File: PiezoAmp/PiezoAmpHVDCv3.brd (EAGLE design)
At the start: 82.5 x 101.3 mm, 35 parts, among them IC1 LM101N, Q1 IRF512, Q2 IRF512, Q3 2N3904, U1 RXX100, X1 MAB32

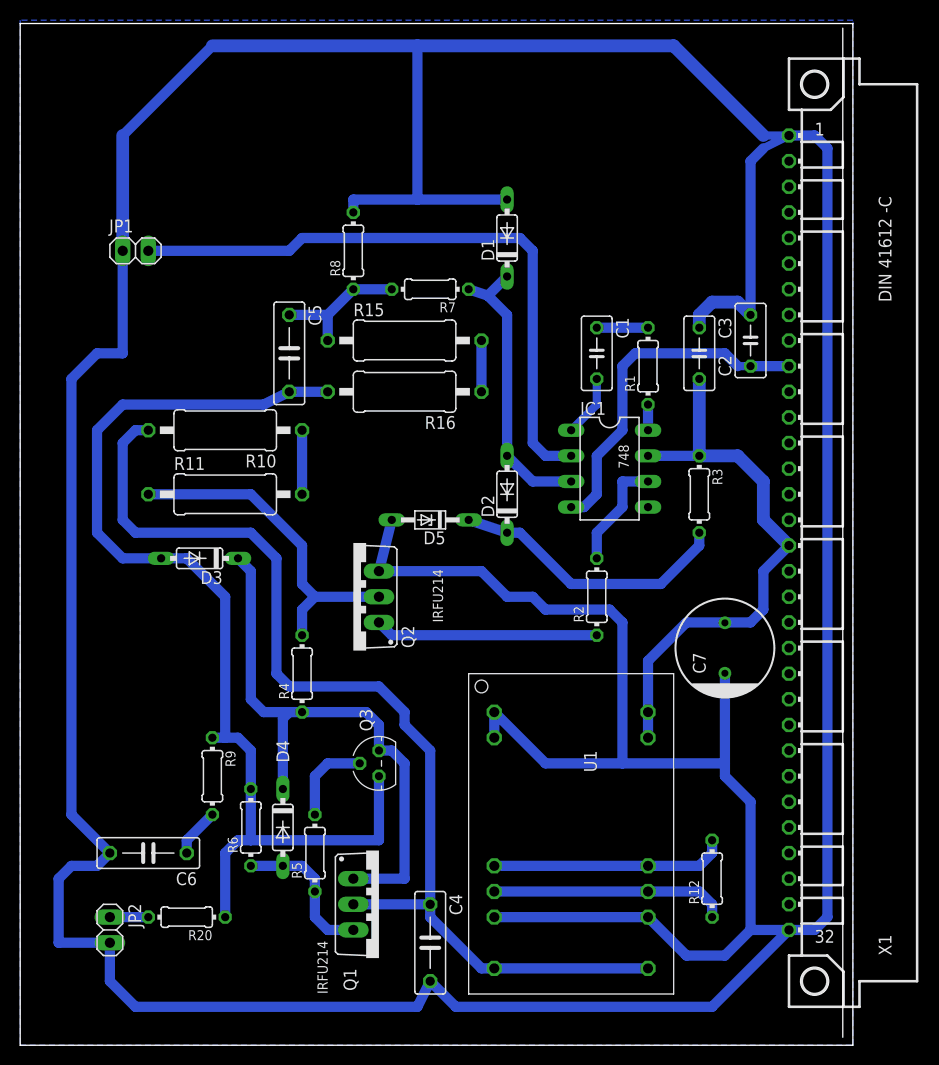
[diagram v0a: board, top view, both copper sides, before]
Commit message: Trying to clean up
Clean up, add Piezo sent to DirtyPCB
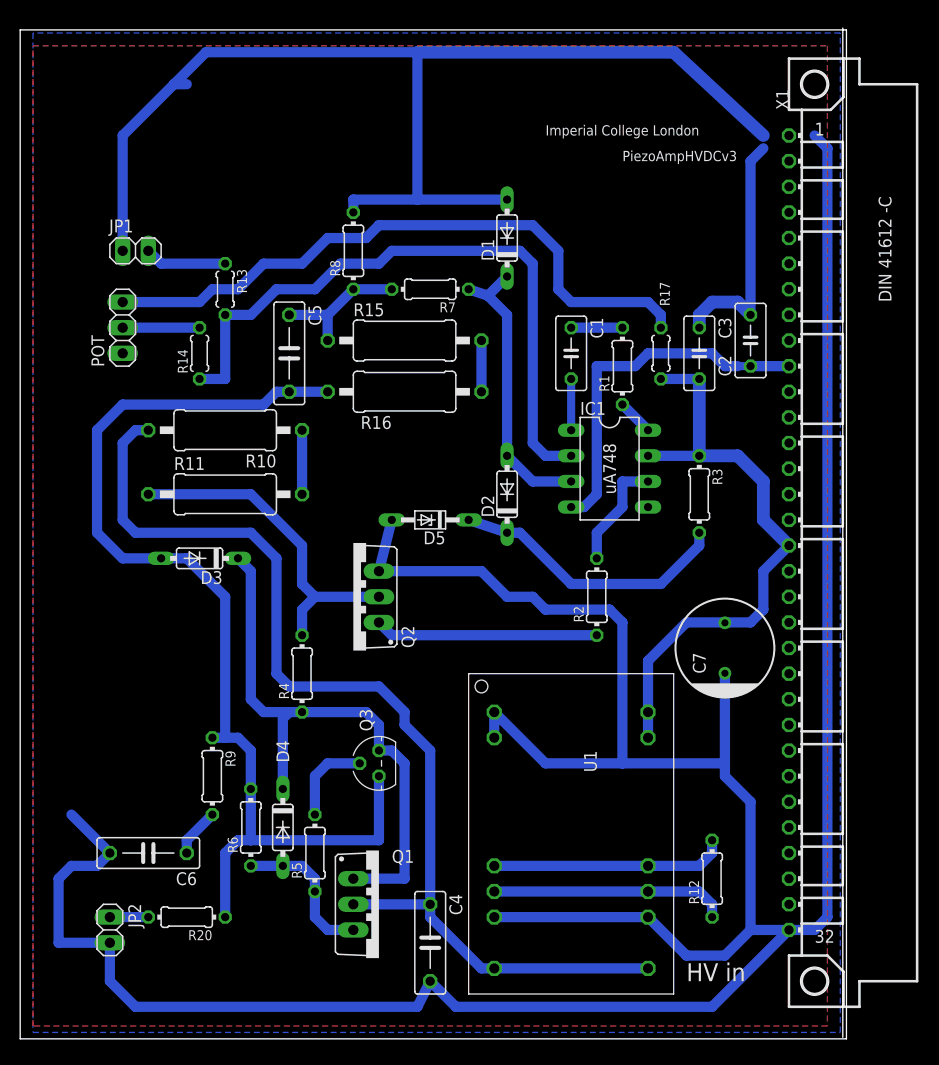
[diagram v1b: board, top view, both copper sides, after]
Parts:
- added POT: 10k, pinhead:1X03
- added R13, R14: 100k, rcl:0204/5
- added R17: 4k7, rcl:0204/5
- D1, D2, D3, D4: value 1N4148DO35-7 -> 1N4148
- Q1, Q2: value IRF512 -> IRFU214
- moved C1 2.54 mm to (132.1, 68.6)
- moved R1 2.54 mm to (137.2, 67.3)
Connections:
- new net N$10: IC1.2, R13.2, R14.1
- new net N$13: POT.2, R14.2
- new net N$17: POT.3, R17.1
- net +15V: now also R17.2
- net GND: now also POT.1
- net N$1: now also R13.1; no longer IC1.2
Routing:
- net GND: track 520.4 -> 452.9 mm
- net N$10: track 0.00 -> 64.6 mm
- net N$17: track 0.00 -> 63.7 mm
- net N$1: track 62.5 -> 8.15 mm
- net N$13: track 0.00 -> 7.62 mm
- net +15V: track 56.1 -> 59.9 mm
- net -15V: track 34.4 -> 35.9 mm
- net N$7: track 2.54 -> 3.59 mm
- net N$27: track 6.13 -> 5.08 mm
- added copper zone on layer 1, net GND
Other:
- board size 82.5 x 101.3 mm -> 81.9 x 100 mm
- board text added: "HV in"
- board text added: "Imperial College London"
- board text added: "PiezoAmpHVDCv3"
- board text added: "uA748"
- board text removed: "748"
- board text removed: "IRFU214"
